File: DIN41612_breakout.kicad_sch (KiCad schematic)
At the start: 4 parts, among them J1 09031967921

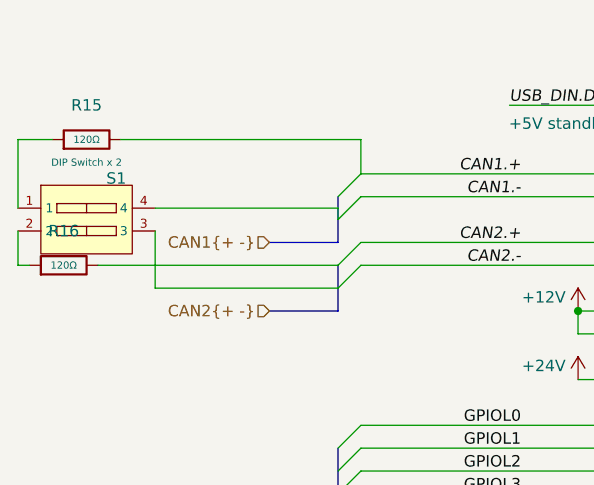
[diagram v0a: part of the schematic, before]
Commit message: Fix paths
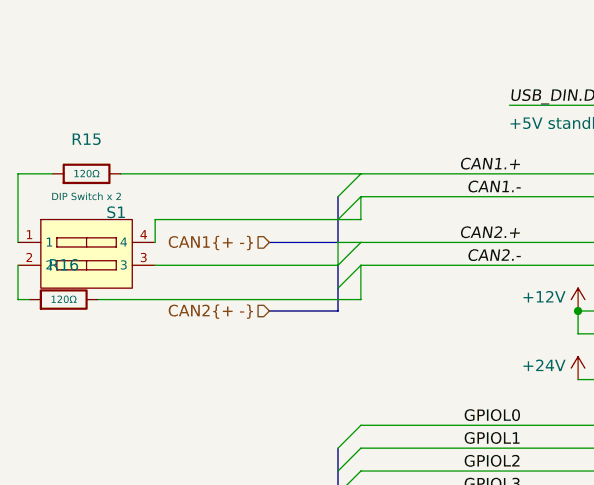
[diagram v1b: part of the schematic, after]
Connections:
- net CAN1.-: now also S1.4
- net CAN2.+: now also S1.3
- net CAN2.-: now also R16.2
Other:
- moved on the sheet: R15, R16, S1
